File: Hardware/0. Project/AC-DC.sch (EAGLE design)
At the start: 0 parts

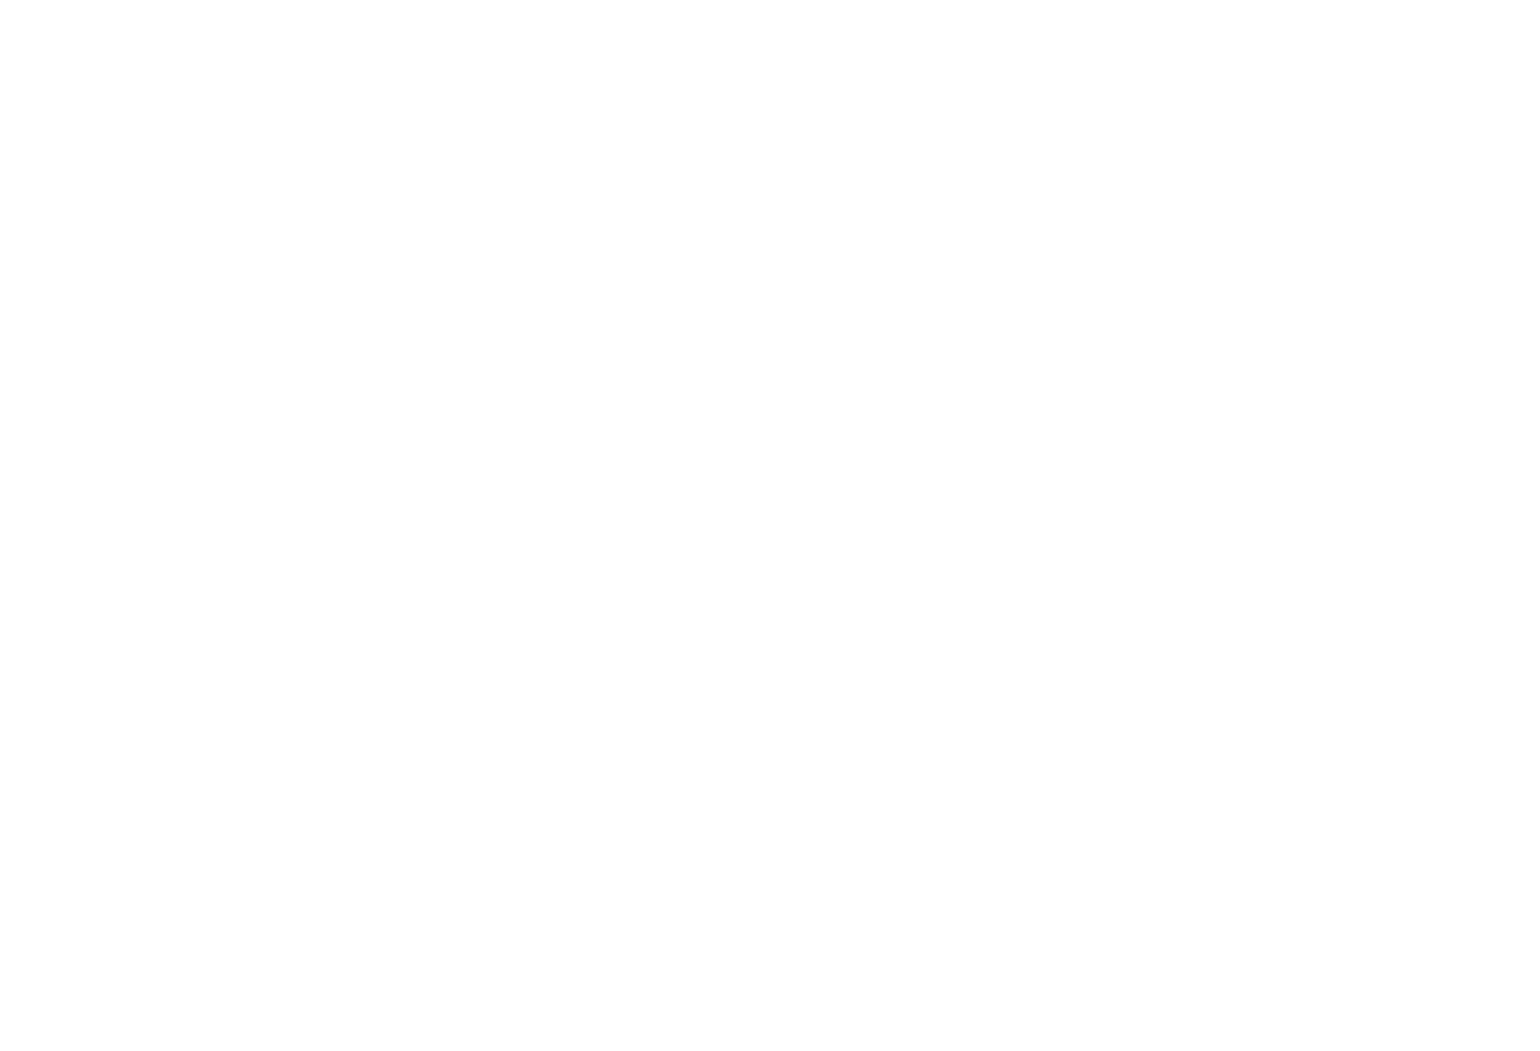
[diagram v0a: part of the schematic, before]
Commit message: Schematic design started
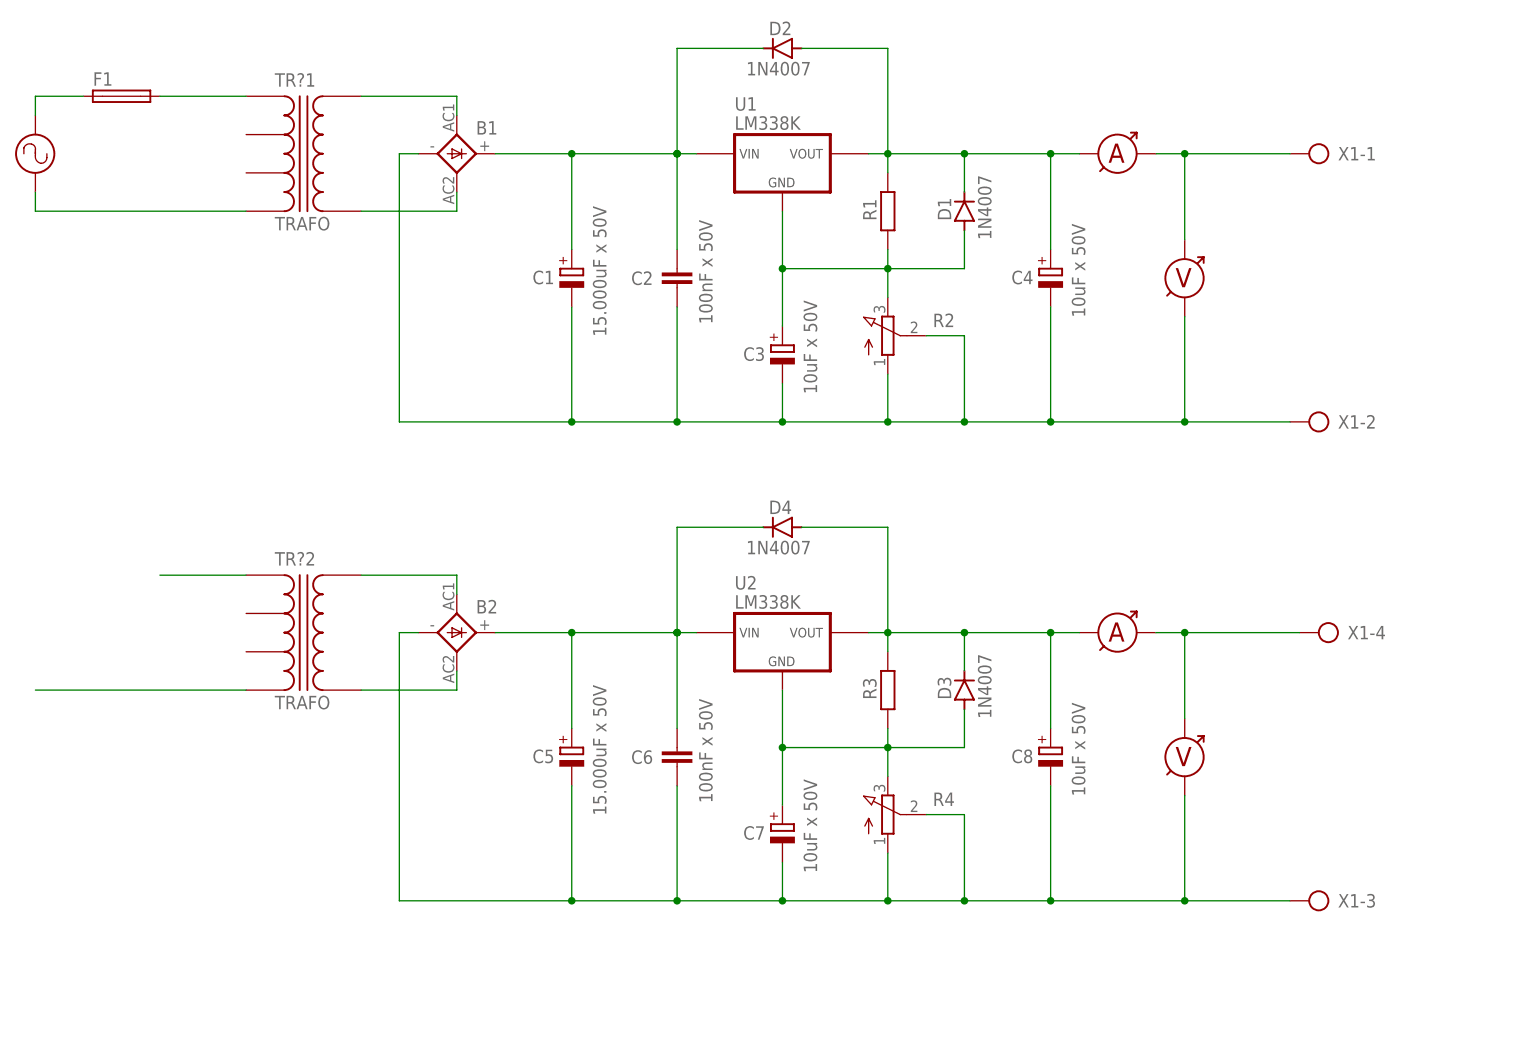
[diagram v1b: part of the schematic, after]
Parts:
- added B1, B2: (no value), rectifier:GBPC1
- added C1, C5: 15.000uF x 50V, rcl:CPOL-EUE10-35
- added C2, C6: 100nF x 50V, rcl:C-EU025-025X050
- added C3, C4, C7, C8: 10uF x 50V, rcl:CPOL-EUE3.5-8
- added D1, D2, D3, D4: 1N4007, diode:1N5060GP
- added F1: (no value), fuse:19559
- added R1, R3: (no value), rcl:R-EU_0207/7
- added R2, R4: (no value), pot:3RP/1610N
- added TR?1, TR?2: TRAFO, Trafo:TRAFO
- added U$1, U$4: AMMETER, Instrumentos:AMMETER
- added U$2, U$5: VOLTMETER, Instrumentos:VOLTMETER
- added U$3: GENERATOR, Instrumentos:GENERATOR
- added U1, U2: LM338K, REG1117:REG1117F
- added X1: (no value), con-ptr500:AK500/4-H
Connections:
- new net N$1: B1.AC1, TR?1.GRN@1
- new net N$10: F1.2, TR?1.BLK@1
- new net N$11: B2.AC1, TR?2.GRN@1
- new net N$12: B2.AC2, TR?2.GRN@2
- new net N$13: B2.+, C5.+, C6.1, D4.C, U2.VIN
- new net N$14: B2.-, C5.-, C6.2, C7.-, C8.-, R4.A, R4.S, U$5.P$2, X1-3.KL
- new net N$15: C8.+, D3.C, D4.A, R3.2, U$4.P$3, U2.VOUT
- new net N$16: C7.+, D3.A, R3.1, R4.E, U2.GND
- new net N$17: U$4.P$2, U$5.P$3, X1-4.KL
- new net N$18: TR?2.GRN/YEL1
- new net N$19: TR?2.BLK@1
- new net N$2: B1.AC2, TR?1.GRN@2
- new net N$3: B1.+, C1.+, C2.1, D2.C, U1.VIN
- new net N$4: B1.-, C1.-, C2.2, C3.-, C4.-, R2.A, R2.S, U$2.P$2, X1-2.KL
- new net N$5: C4.+, D1.C, D2.A, R1.2, U$1.P$3, U1.VOUT
- new net N$6: C3.+, D1.A, R1.1, R2.E, U1.GND
- new net N$7: U$1.P$2, U$2.P$3, X1-1.KL
- new net N$8: F1.1, U$3.P$3
- new net N$9: TR?1.GRN/YEL1, U$3.P$2
